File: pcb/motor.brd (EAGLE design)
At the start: 44.4 x 77.8 mm, 11 parts, among them Q1 IRF3708, Q2 IRF3708

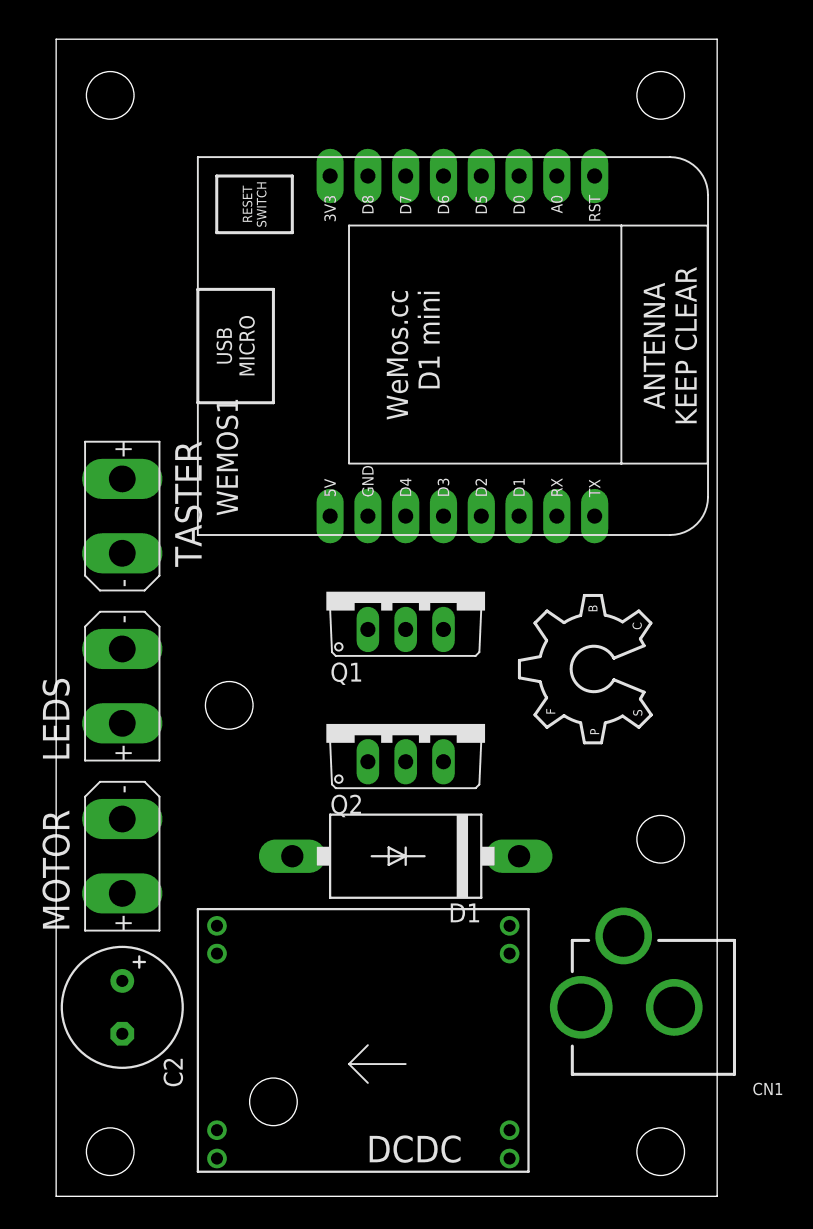
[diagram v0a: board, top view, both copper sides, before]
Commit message: first version of motor driver pcb layout
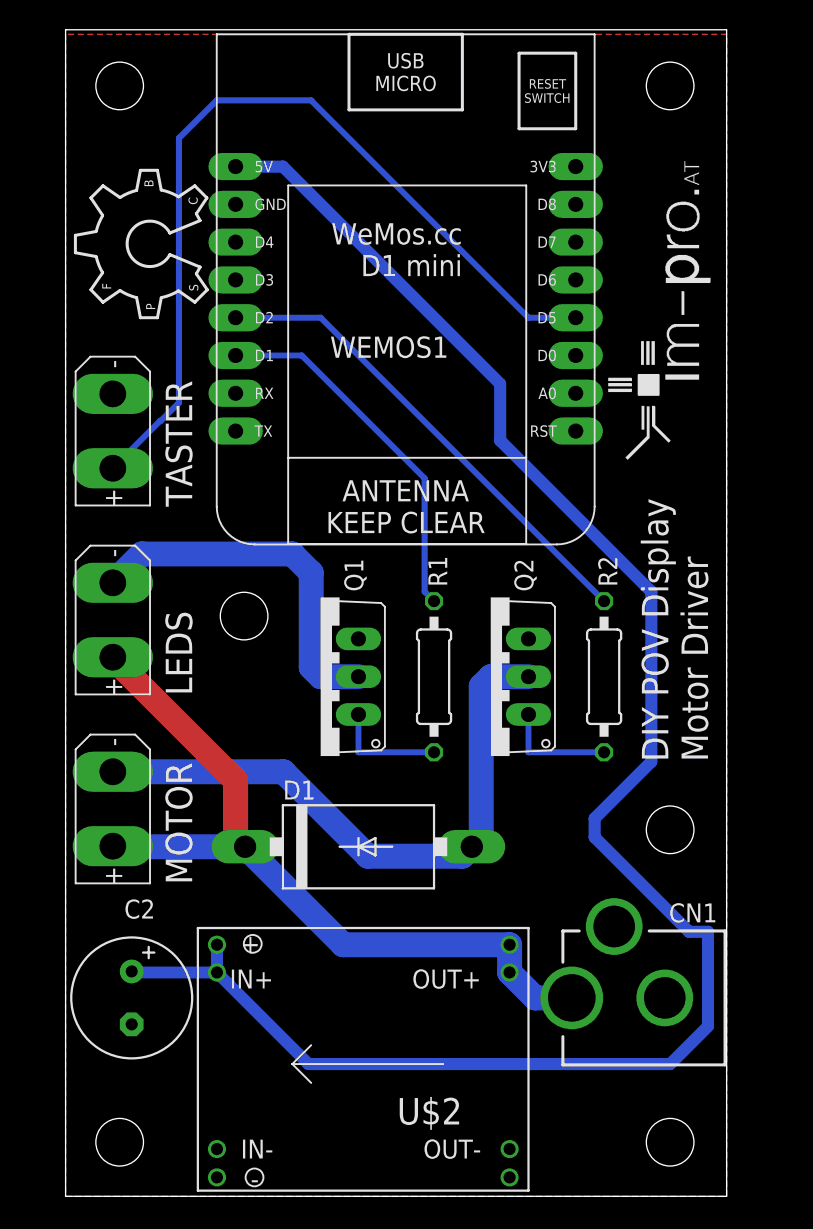
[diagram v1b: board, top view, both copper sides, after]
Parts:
- removed DCDC: DCDC, main:DCDC
- added R1, R2: 180R, rcl:0207/10
- added U$1: LOGO20MM, im-pro-logo:LOGO_20MM
- added U$2: DCDC_5V, diypov:DCDC
- C2: value (none) -> 100u
- moved LOGO1 41.3 mm to (9.53, 59.1)
- moved Q1 8.08 mm to (17.1, 34.9), turned to 90 degrees
- moved Q2 6.54 mm to (28.6, 34.9), turned to 90 degrees
- moved TASTER 5.75 mm to (3.17, 51.4), turned to 90 degrees
- moved LEDS 4.49 mm to (3.17, 38.7)
- moved WEMOS1 3.86 mm to (24.1, 59.1), turned to 180 degrees
- moved D1 3.24 mm to (19.7, 23.5), turned to 0 degrees
- moved MOTOR 3.24 mm to (3.17, 26.0)
- moved C2 0.90 mm to (4.45, 13.3)
- moved CN1 0.90 mm to (47.6, 13.3)
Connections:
- new net N$6: Q2.1, R2.2
- new net N$7: Q1.1, R1.2
- net +12V: now also U$2.VIN1, U$2.VIN2; no longer DCDC.VIN1, DCDC.VIN2
- net +5V: now also U$2.VOUT1, U$2.VOUT2; no longer DCDC.VOUT1, DCDC.VOUT2
- net GND: now also U$2.GND1, U$2.GND2, U$2.GND3, U$2.GND4; no longer DCDC.GND1, DCDC.GND2, DCDC.GND3, DCDC.GND4
- net N$3: now also R1.1; no longer Q1.1
- net N$5: now also R2.1; no longer Q2.1
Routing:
- net +5V: track 0.00 -> 120.9 mm
- net N$4: track 0.00 -> 57.8 mm
- net +12V: track 0.00 -> 53.0 mm
- net N$1: track 0.00 -> 41.2 mm
- net N$5: track 0.00 -> 32.7 mm
- net N$3: track 0.00 -> 24.6 mm
- net N$2: track 0.00 -> 24.5 mm
- net N$7: track 0.00 -> 7.62 mm
- net N$6: track 0.00 -> 7.62 mm
- added copper zone on layer 1, net GND
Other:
- board size 44.4 x 77.8 mm -> 44.4 x 78.4 mm
- board text added: "DIY POV Display Motor Driver"
